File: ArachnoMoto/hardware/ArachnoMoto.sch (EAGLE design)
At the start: 31 parts, among them J1 PINHEAD-17-REV, J2 PINHEAD-17-REV, U1 DRV8801, U2 DRV8801, U3 USD-SOCKETNEW, X1 1751248, X2 1751248, X3 1751248, X4 1751248

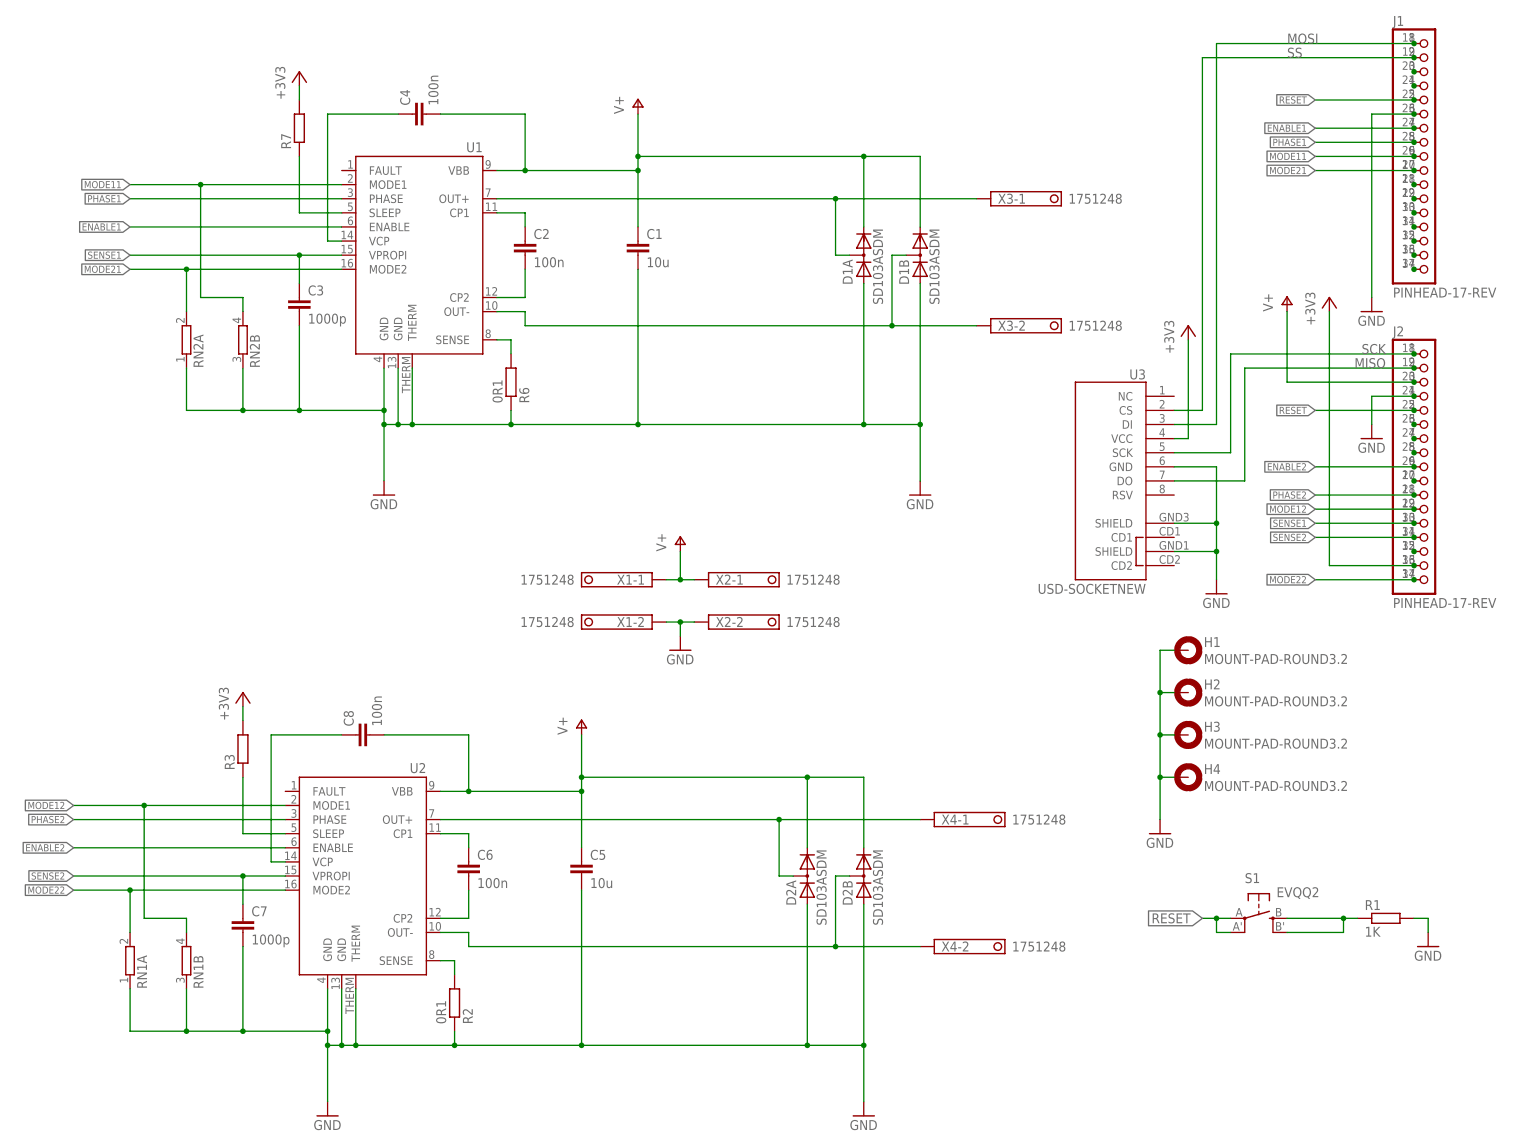
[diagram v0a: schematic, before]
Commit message: Ombnibus commit because I am not sure what I did...
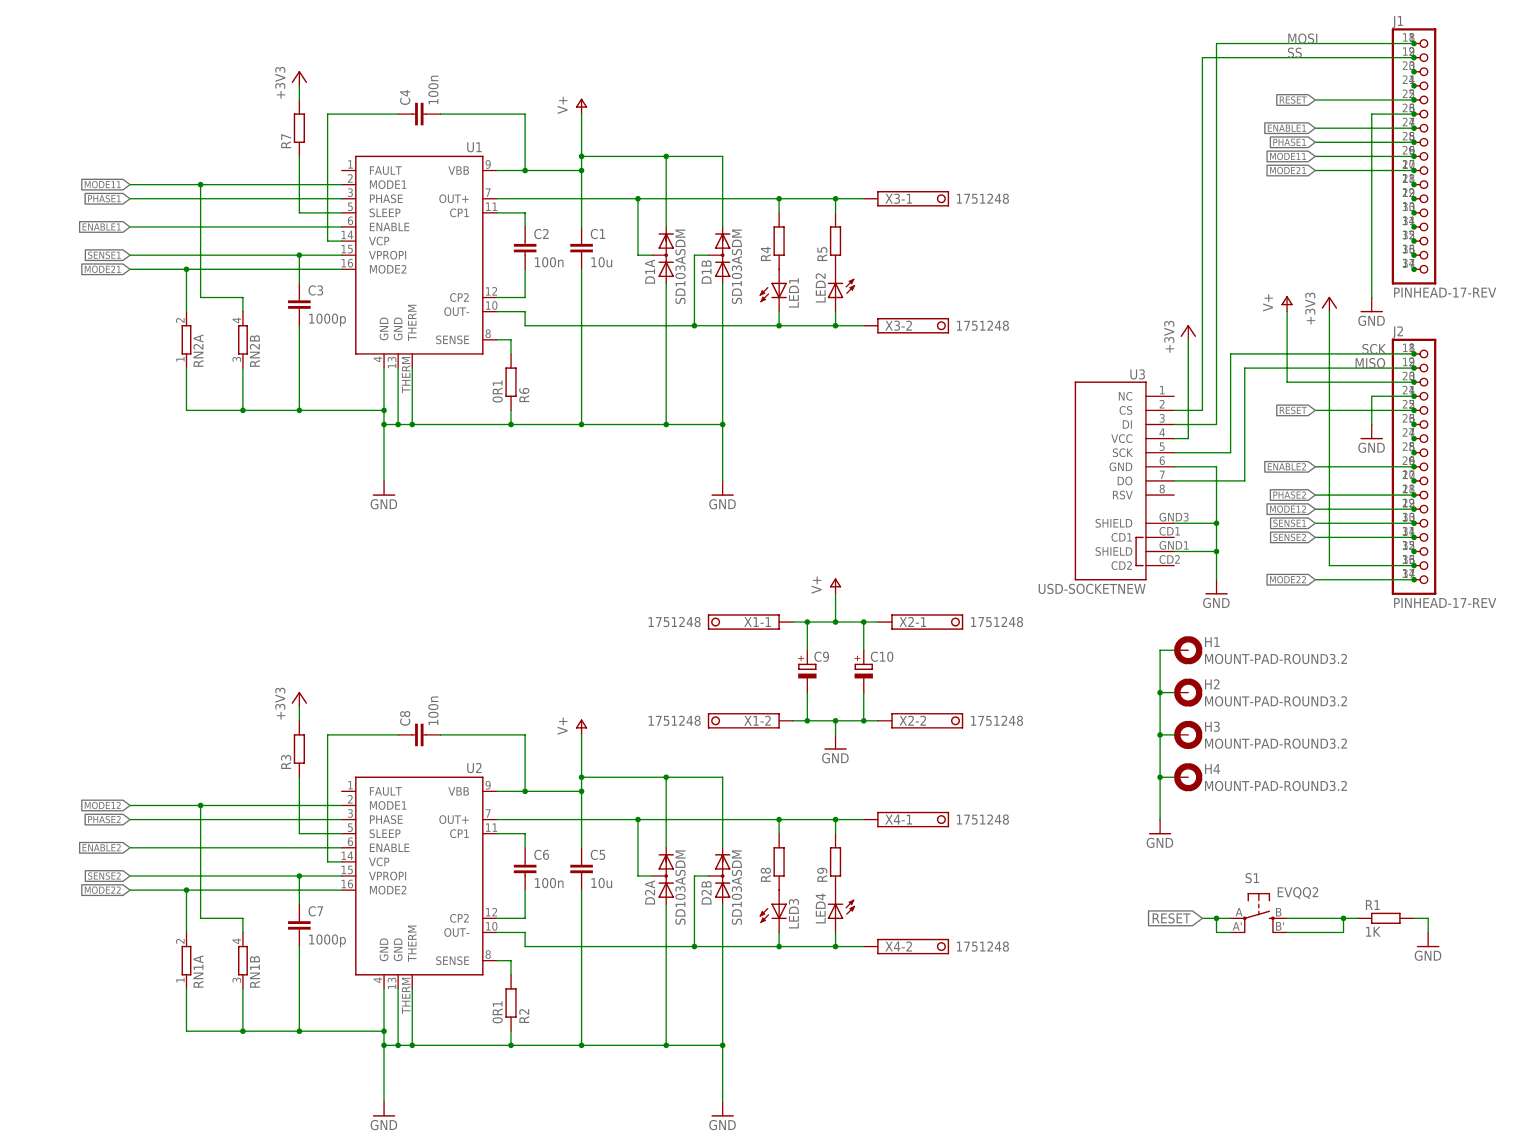
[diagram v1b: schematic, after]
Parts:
- added C10, C9: (no value), resistor:CPOL-EUE5-10.5
- added LED1, LED2, LED3, LED4: (no value), adafruit:LEDCHIP-LED0603
- added R4, R5, R8, R9: (no value), resistor:R-EU_R0603
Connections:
- new net N$11: LED2.C, R5.1
- new net N$12: LED3.A, R8.1
- new net N$14: LED4.C, R9.1
- new net N$4: LED1.A, R4.1
- net GND: now also C10.-, C9.-
- net N$1: now also R8.2, R9.2
- net N$18: now also R4.2, R5.2
- net N$19: now also LED1.C, LED2.A
- net N$3: now also LED3.C, LED4.A
- net V+: now also C10.+, C9.+
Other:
- moved on the sheet: C1, C6, C7, C8, D1A, D1B, D2A, D2B, R2, R3, RN1A, RN1B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
